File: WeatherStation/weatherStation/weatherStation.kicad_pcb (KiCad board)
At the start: 2 copper layers, 60.7 x 36.9 mm, 67 parts, among them J1 RJ12, J2 Conn_01x03, J3 AVR-ISP-6, J4 USB_B_Micro, J5 Conn_01x02, J6 Conn_01x04, Q1 AO4430, SW1 SW_Push, SW2 SW_SPDT, U1 ATmega328P-AU, U10 MAX40200, U11 MAX17048, U12 LM3671, U13 BQ24210, U2 ATtiny45V-10PU, U3 BME280, U4 FDW254p, U5 FT230XS, U6 MB85RC64, U7 DS3231_Breakout, U8 BQ297xy, U9 ECH8693R, Y1 Crystal

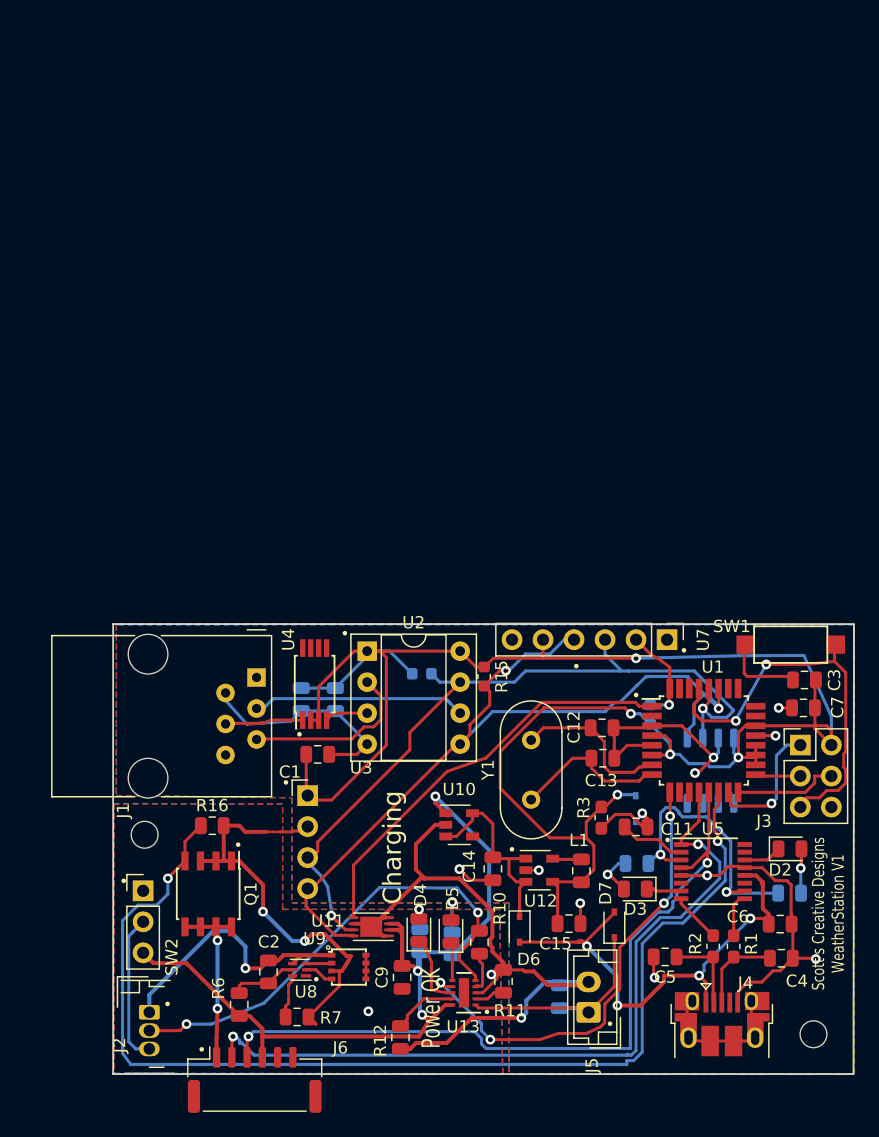
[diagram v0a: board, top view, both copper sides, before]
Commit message: commit before more
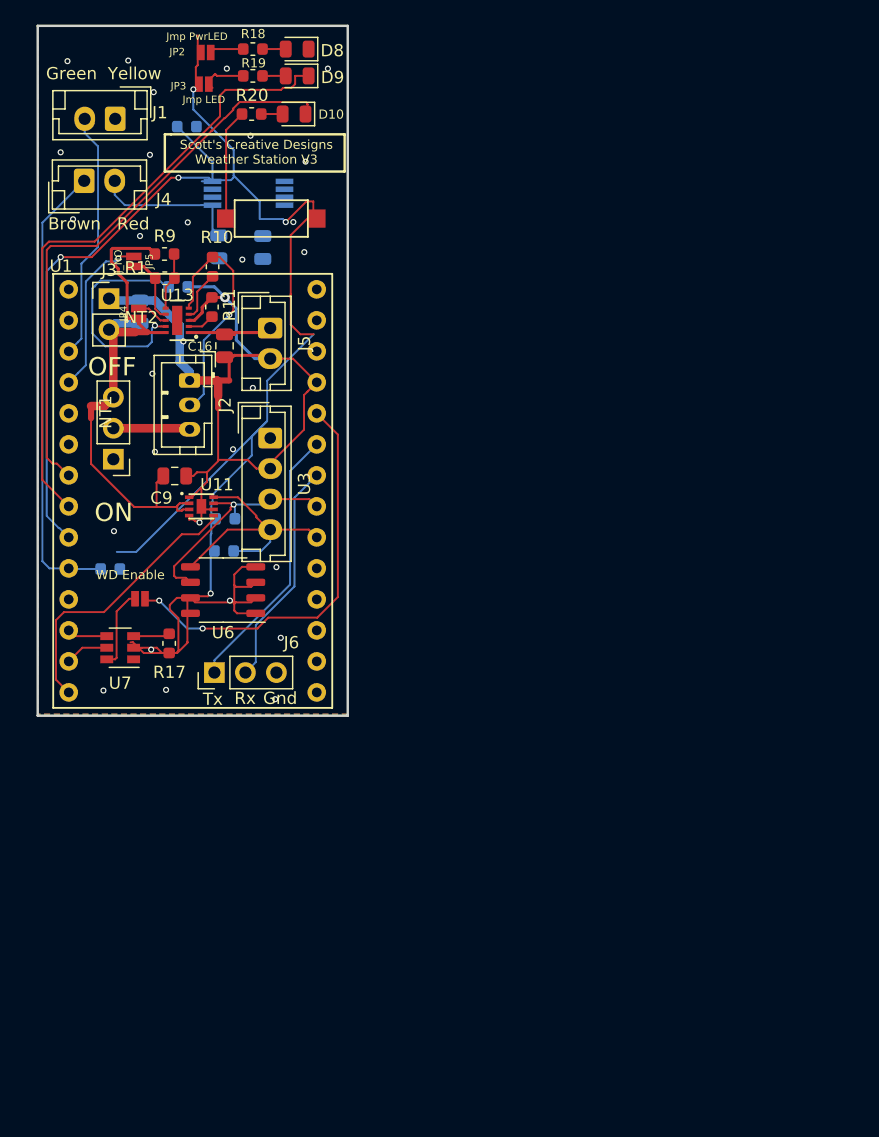
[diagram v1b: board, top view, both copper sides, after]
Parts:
- removed C10, C11, C3, C6, C7, C8: 100nF, Capacitor_SMD:C_0805_2012Metric
- removed C12, C13: 22nF, Capacitor_SMD:C_0805_2012Metric
- removed C14: 4.7uF, Capacitor_SMD:C_0805_2012Metric
- removed C15: 10uF, Capacitor_SMD:C_0805_2012Metric
- removed C4, C5: 47pF, Capacitor_SMD:C_0805_2012Metric
- removed D1: D, Diode_SMD:D_SOD-323
- removed D2: TXLED, LED_SMD:LED_0805_2012Metric
- removed D3: RXLED, LED_SMD:LED_0805_2012Metric
- removed D4, D5: LED, LED_SMD:LED_0805_2012Metric
- removed D6, D7: D_Schottky, Diode_SMD:D_SOD-323
- removed L1: 2.2uH, Inductor_SMD:L_0805_2012Metric
- removed Q1: AO4430, Package_SO:SOIC-8_3.9x4.9mm_P1.27mm
- removed R16, R6, R8: 330, Resistor_SMD:R_0805_2012Metric
- removed R2: 27R, Resistor_SMD:R_0603_1608Metric_Pad1.05x0.95mm_HandSolder
- removed R3: 100k, Resistor_SMD:R_0603_1608Metric_Pad1.05x0.95mm_HandSolder
- removed R4, R5: 270R, Resistor_SMD:R_0805_2012Metric
- removed R7: 2.2k, Resistor_SMD:R_0805_2012Metric
- removed REF** (x2): MountingHole_2.2mm_M2, MountingHole:MountingHole_2.2mm_M2
- removed SW1: SW_Push, EbayParts:Tact_SMD_Switch
- removed U10: MAX40200, Package_TO_SOT_SMD:SOT-23-5
- removed U12: LM3671, Package_TO_SOT_SMD:SOT-23-5
- removed U2: ATtiny45V-10PU, Package_DIP:DIP-8_W7.62mm_Socket
- removed U5: FT230XS, Package_SO:SSOP-16_3.9x4.9mm_P0.635mm
- removed U8: BQ297xy, Package_SON:WSON-6_1.5x1.5mm_P0.5mm
- removed U9: ECH8693R, CustomFP:sot-28
- removed W1, W3: Wire_Jump, CustomFP:wireJump
- removed Y1: Crystal, Crystal:Crystal_HC49-U_Vertical
- added C18: 100nF, Capacitor_SMD:C_0805_2012Metric, B.Cu at (107.5, 70.2)
- added D10: GPLED, LED_SMD:LED_0805_2012Metric, F.Cu at (113.7, 59.3)
- added D8: 3V3 OK, LED_SMD:LED_0805_2012Metric, F.Cu at (114.0, 54.0)
- added D9: GPLED, LED_SMD:LED_0805_2012Metric, F.Cu at (114.0, 56.2)
- added JP1: Jmp_NO, Jumpers:SMT-JUMPER_2_NO_NO-SILK, F.Cu at (101.1, 99.0)
- added JP2: Jmp PwrLED, Jumpers:SMT-JUMPER_2_NO_NO-SILK, F.Cu at (106.5, 54.3)
- added JP3: Jmp LED, Jumpers:SMT-JUMPER_2_NO_NO-SILK, F.Cu at (106.3, 56.8)
- added JP4: J_NO, Jumpers:SMT-JUMPER_2_NO_NO-SILK, F.Cu at (101.0, 75.6)
- added JP5: J_NO, Jumpers:SMT-JUMPER_2_NO_NO-SILK, F.Cu at (100.6, 71.4)
- added NT1: Net-Tie_2, NetTie:NetTie-2_SMD_Pad0.5mm, F.Cu at (97.1, 83.7)
- added NT2: Net-Tie_2, NetTie:NetTie-2_SMD_Pad0.5mm, F.Cu at (101.2, 77.2)
- added NT3: Net-Tie_2, NetTie:NetTie-2_SMD_Pad0.5mm, F.Cu at (107.9, 81.1)
- added NT4: Net-Tie_2, NetTie:NetTie-2_SMD_Pad0.5mm, F.Cu at (107.5, 82.9)
- added R17: 33k, Resistor_SMD:R_0603_1608Metric, F.Cu at (103.5, 102.7)
- added R18: 300, Resistor_SMD:R_0603_1608Metric, F.Cu at (110.3, 54.0)
- added R19: 300, Resistor_SMD:R_0603_1608Metric, F.Cu at (110.3, 56.2)
- added R20: 300, Resistor_SMD:R_0603_1608Metric, F.Cu at (110.2, 59.3)
- added R25: 10k, Resistor_SMD:R_0603_1608Metric, B.Cu at (98.7, 96.6)
- added SW3: LED_Push, EbayParts:Tact_SMD_Switch, F.Cu at (114.8, 66.4)
- C1, R15, U4: moved to B.Cu
- C16: value 0.1uF -> 1uF; moved to F.Cu
- C2: value 0.1uF -> 1uF; moved to B.Cu
- J1: value RJ12 -> Conn_01x02; footprint Connector_RJ:RJ12_Amphenol_54601 -> Connector_JST:JST_EH_B02B-EH-A_1x02_P2.50mm_Vertical
- J2: footprint CustomFP:JST_EH_B03B-EH-A_1x03_P1.50mm_Vertical -> Connector_JST:JST_PH_B3B-PH-K_1x03_P2.00mm_Vertical
- J3: value AVR-ISP-6 -> Conn_01x02_Female; footprint Connector_PinHeader_2.54mm:PinHeader_2x03_P2.54mm_Vertical -> Connector_PinHeader_2.54mm:PinHeader_1x02_P2.54mm_Vertical
- J4: value USB_B_Micro -> Conn_01x02; footprint Connector_USB:USB_Micro-B_Amphenol_10103594-0001LF_Horizontal -> Connector_JST:JST_EH_B02B-EH-A_1x02_P2.50mm_Vertical
- J6: value Conn_01x04 -> Conn_01x03_Female; footprint Connector_JST:JST_GH_SM06B-GHS-TB_1x06-1MP_P1.25mm_Horizontal -> Connector_PinHeader_2.54mm:PinHeader_1x03_P2.54mm_Vertical
- R1: value 27R -> 10k; footprint Resistor_SMD:R_0603_1608Metric_Pad1.05x0.95mm_HandSolder -> Resistor_SMD:R_0603_1608Metric
- R10: footprint Resistor_SMD:R_0805_2012Metric -> Resistor_SMD:R_0603_1608Metric
- R11: value 330 -> 750; footprint Resistor_SMD:R_0805_2012Metric -> Resistor_SMD:R_0603_1608Metric
- R12: footprint Resistor_SMD:R_0805_2012Metric -> Resistor_SMD:R_0603_1608Metric; moved to B.Cu
- R13: value 50k -> 10k
- R9: value 330 -> 100k; footprint Resistor_SMD:R_0805_2012Metric -> Resistor_SMD:R_0603_1608Metric; moved to F.Cu
- U1: value ATmega328P-AU -> MKRGSM1400; footprint Package_QFP:TQFP-32_7x7mm_P0.8mm -> CustomFP:MKRGSM1400
- U11: footprint Package_DFN_QFN:TDFN-8-1EP_3x2mm_P0.5mm_EP1.80x1.65mm -> CustomFP:TQFN-8_2x2x0.75
- U3: footprint CustomFP:PinHeader_1x04_P2.54mm_Horizontal -> Connector_JST:JST_EH_B04B-EH-A_1x04_P2.50mm_Vertical
- U6: moved to F.Cu
- U7: value DS3231_Breakout -> TPL5010; footprint Connector_PinHeader_2.54mm:PinHeader_1x06_P2.54mm_Vertical -> Package_TO_SOT_SMD:SOT-23-6
- moved J4 86.6 mm to (96.5, 64.8)
- moved R1 71.9 mm to (103.1, 72.7), turned to 180 degrees
- moved J3 67.4 mm to (98.6, 74.4)
- moved R12 64.1 mm to (104.2, 73.5), turned to 0 degrees
- moved U1 62.8 mm to (96.5, 73.7)
- moved J5 61.8 mm to (111.8, 76.8), turned to 270 degrees
- moved R13 61.3 mm to (104.9, 60.3), turned to 180 degrees
- moved R9 61.2 mm to (103.1, 70.8), turned to 0 degrees
- moved R11 60.2 mm to (107.0, 75.1)
- moved C16 60.0 mm to (108.0, 78.3), turned to 270 degrees
- moved U13 59.9 mm to (104.1, 76.2)
- moved R10 59.5 mm to (107.0, 71.8), turned to 90 degrees
- moved C2 55.1 mm to (101.1, 75.5)
- moved J2 51.9 mm to (105.2, 81.1)
- moved J1 47.2 mm to (99.1, 59.7), turned to 180 degrees
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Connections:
- net Net-(J2-Pad3) renamed /Sheet5C1E5C91/Batt_int
- C16 pad 2: /Sheet5C1E5C91/Pack- -> GND
- C2 pad 1: Net-(C2-Pad1) -> /Sheet5C1E5C91/Batt+
- C2 pad 2: /Sheet5C1E5C91/Batt- -> GND
- C9 pad 1: /Sheet5C1E5C91/Pack- -> GND
- C9 pad 2: /Sheet5C1E5C91/Batt+ -> /Sheet5C1E5C91/BattMon+
- J1 pad 1: (no net) -> GND
- J1 pad 2: GND -> /ANE_Pulse
- J2 pad 1: /Sheet5C1E5C91/Batt- -> GND
- J3 pad 1: /MISO -> GND
- J3 pad 2: 3V3 -> /Sheet5C1E5C91/Batt+
- J4 pad 1: USB_PWR -> /ANE_Tx
- J4 pad 2: Net-(C5-Pad1) -> /ANE_Vcc
- J5 pad 2: /Sheet5C1E5C91/Pack- -> GND
- J6 pad 1: /Sheet5C1E5C91/SIM- -> Net-(J6-Pad1)
- J6 pad 2: Rx -> Net-(J6-Pad2)
- J6 pad 3: Tx -> GND
- R1 pad 2: Net-(C4-Pad1) -> Net-(JP5-Pad2)
- R10 pad 1: /Sheet5C1E5C91/NTC -> Net-(R10-Pad1)
- R10 pad 2: Net-(R10-Pad2) -> /Sheet5C1E5C91/NTC
- R11 pad 2: /Sheet5C1E5C91/Pack- -> GND
- R12 pad 2: /Sheet5C1E5C91/Pack- -> GND
- R13 pad 2: /RTC_INT -> /ANE_Vcc_EN
- R9 pad 1: /Sheet5C1E5C91/Batt+ -> /Sheet5C1E5C91/Batt_Chrg+
- R9 pad 2: Net-(D5-Pad2) -> Net-(R1-Pad1)
- SW2 pad 1: (no net) -> Net-(SW2-Pad1)
- U1 pad 1: BATT_ALRT -> Net-(U1-Pad1)
- U1 pad 10: (no net) -> /ANE_Tx
- U1 pad 11: (no net) -> Net-(U1-Pad11)
- U1 pad 12: Rx -> /DONE
- U1 pad 13: Tx -> /WAKE
- U1 pad 14: SIM_EN -> BATT_ALRT
- U1 pad 15: /MISO -> Net-(U1-Pad15)
- U1 pad 16: /MOSI -> Net-(U1-Pad16)
- U1 pad 17: /SCK -> Net-(U1-Pad17)
- U1 pad 18: 3V3 -> Net-(U1-Pad18)
- U1 pad 19: 3V3 -> Net-(U1-Pad19)
- U1 pad 2: (no net) -> Net-(U1-Pad2)
- U1 pad 20: 3V3 -> I2C_SDA
- U1 pad 21: GND -> I2C_SCL
- U1 pad 22: 3V3 -> Net-(J6-Pad2)
- U1 pad 23: (no net) -> Net-(J6-Pad1)
- U1 pad 24: (no net) -> /RESET
- U1 pad 25: (no net) -> GND
- U1 pad 26: (no net) -> 3V3
- U1 pad 27: I2C_SDA -> Net-(U1-Pad27)
- U1 pad 28: I2C_SCL -> Net-(U1-Pad28)
- U1 pad 3: GND -> /ANE_Pulse
- U1 pad 4: 3V3 -> CHRG_EN
- U1 pad 5: GND -> Net-(U1-Pad5)
- U1 pad 6: 3V3 -> Net-(U1-Pad6)
- U1 pad 7: /XTAL1 -> /GPLED2
- U1 pad 8: /XTAL2 -> /GPLED1
- U1 pad 9: Charge_EN -> /ANE_Vcc_EN
- U11 pad 1: /Sheet5C1E5C91/Pack- -> GND
- U11 pad 2: /Sheet5C1E5C91/Batt+ -> /Sheet5C1E5C91/BattMon+
- U11 pad 3: /Sheet5C1E5C91/Batt+ -> /Sheet5C1E5C91/BattMon+
- U11 pad 4: /Sheet5C1E5C91/Pack- -> GND
- U11 pad 6: /Sheet5C1E5C91/Pack- -> GND
- U11 pad 9: /Sheet5C1E5C91/Pack- -> GND
- U13 pad 10: /Sheet5C1E5C91/Batt+ -> /Sheet5C1E5C91/Batt_Chrg+
- U13 pad 3: /Sheet5C1E5C91/Pack- -> GND
- U13 pad 4: Net-(R10-Pad2) -> Net-(R10-Pad1)
- U13 pad 6: Net-(D5-Pad1) -> Net-(R1-Pad1)
- U13 pad 7: Charge_EN -> Net-(JP5-Pad2)
- U4 pad 5: (no net) -> Net-(U4-Pad5)
- U4 pad 6: (no net) -> Net-(U4-Pad6)
- U4 pad 7: (no net) -> Net-(U4-Pad7)
- U4 pad 8: (no net) -> Net-(U4-Pad8)
- U7 pad 1: (no net) -> 3V3
- U7 pad 2: /RTC_INT -> GND
- U7 pad 3: I2C_SCL -> Net-(R17-Pad2)
- U7 pad 4: I2C_SDA -> /DONE
- U7 pad 5: 3V3 -> /WAKE
- U7 pad 6: GND -> Net-(JP1-Pad1)
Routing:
- net 3V3: track 165.4 -> 40.2 mm, vias 5 -> 2
- net /Sheet5C1E5C91/Pack-: track 93.8 -> 0.00 mm, vias 5 -> 0
- net SIM_EN: track 91.4 -> 0.00 mm, vias 2 -> 0
- net GND: track 80.0 -> 146.7 mm, vias 10 -> 31
- net Rx: track 63.8 -> 0.00 mm, vias 2 -> 0
- net Tx: track 61.1 -> 0.00 mm, vias 2 -> 0
- net /Sheet5C1E5C91/Batt+: track 69.4 -> 12.8 mm, vias 3 -> 0
- net /GPLED1: track 0.00 -> 51.1 mm
- net I2C_SDA: track 70.2 -> 22.0 mm, vias 2 -> 0
- net /GPLED2: track 0.00 -> 47.0 mm
- net I2C_SCL: track 64.0 -> 19.6 mm, vias 2 -> 1
- net /ANE_Vcc_EN: track 3.56 -> 46.0 mm, vias 0 -> 2
- net USB_PWR: track 39.8 -> 0.00 mm, vias 4 -> 0
- net Charge_EN: track 38.4 -> 0.00 mm, vias 4 -> 0
- net /ANE_Tx: track 13.8 -> 37.6 mm
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- removed copper zone on B.Cu, net /Sheet5C1E5C91/Pack-
- removed copper zone on F.Cu, net /Sheet5C1E5C91/Pack-
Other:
- board size 60.7 x 36.9 mm -> 25.4 x 56.5 mm
- net class BattPwr: trace_width 0.33 -> 0.7
- net class SmallSig added: clearance 0.2, trace_width 0.16, via_dia 0.5, via_drill 0.3
- rule trace_min: 0.2 -> 0.127
- rule via_min_size: 0.4 -> 0.45
- board text added: "Brown Red"
- board text added: "Gnd"
- board text added: "Green Yellow"
- board text added: "OFF"
- board text added: "ON"
- board text added: "Rx"
- board text added: "Scott's Creative Designs Weather Station V3"
- board text added: "Tx"
- board text added: "WD Enable"
- board text removed: "Charging"
- board text removed: "Power OK"
- board text removed: "Scott's Creative Designs WeatherStation V1"
